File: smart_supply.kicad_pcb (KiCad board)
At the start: 2 copper layers, 40 x 40 mm, 26 parts, among them J2 Conn_01x05_Pin, J3 Conn_01x02_Pin, J4 Conn_01x06_Pin, J5 Conn_01x06_Pin, U5 ADE7953xCP, U7 MCP1825ST-3302E/DB, Y1 3.58M

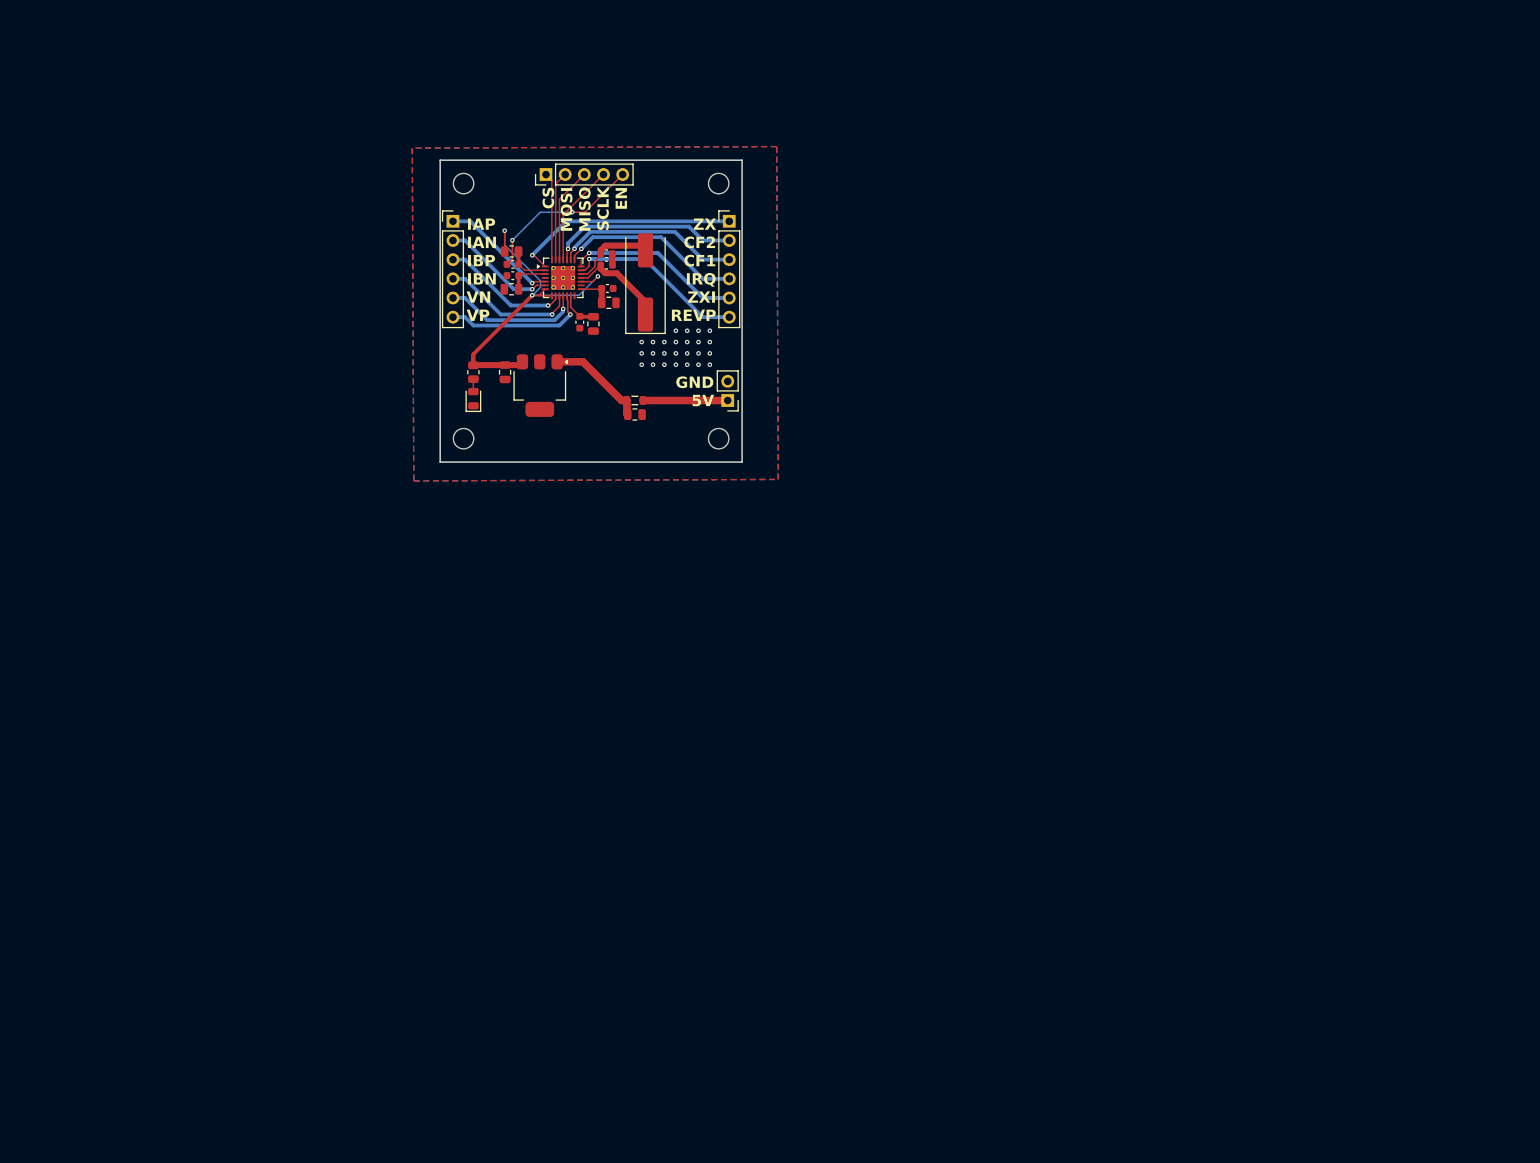
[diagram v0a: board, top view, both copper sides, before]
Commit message: created board
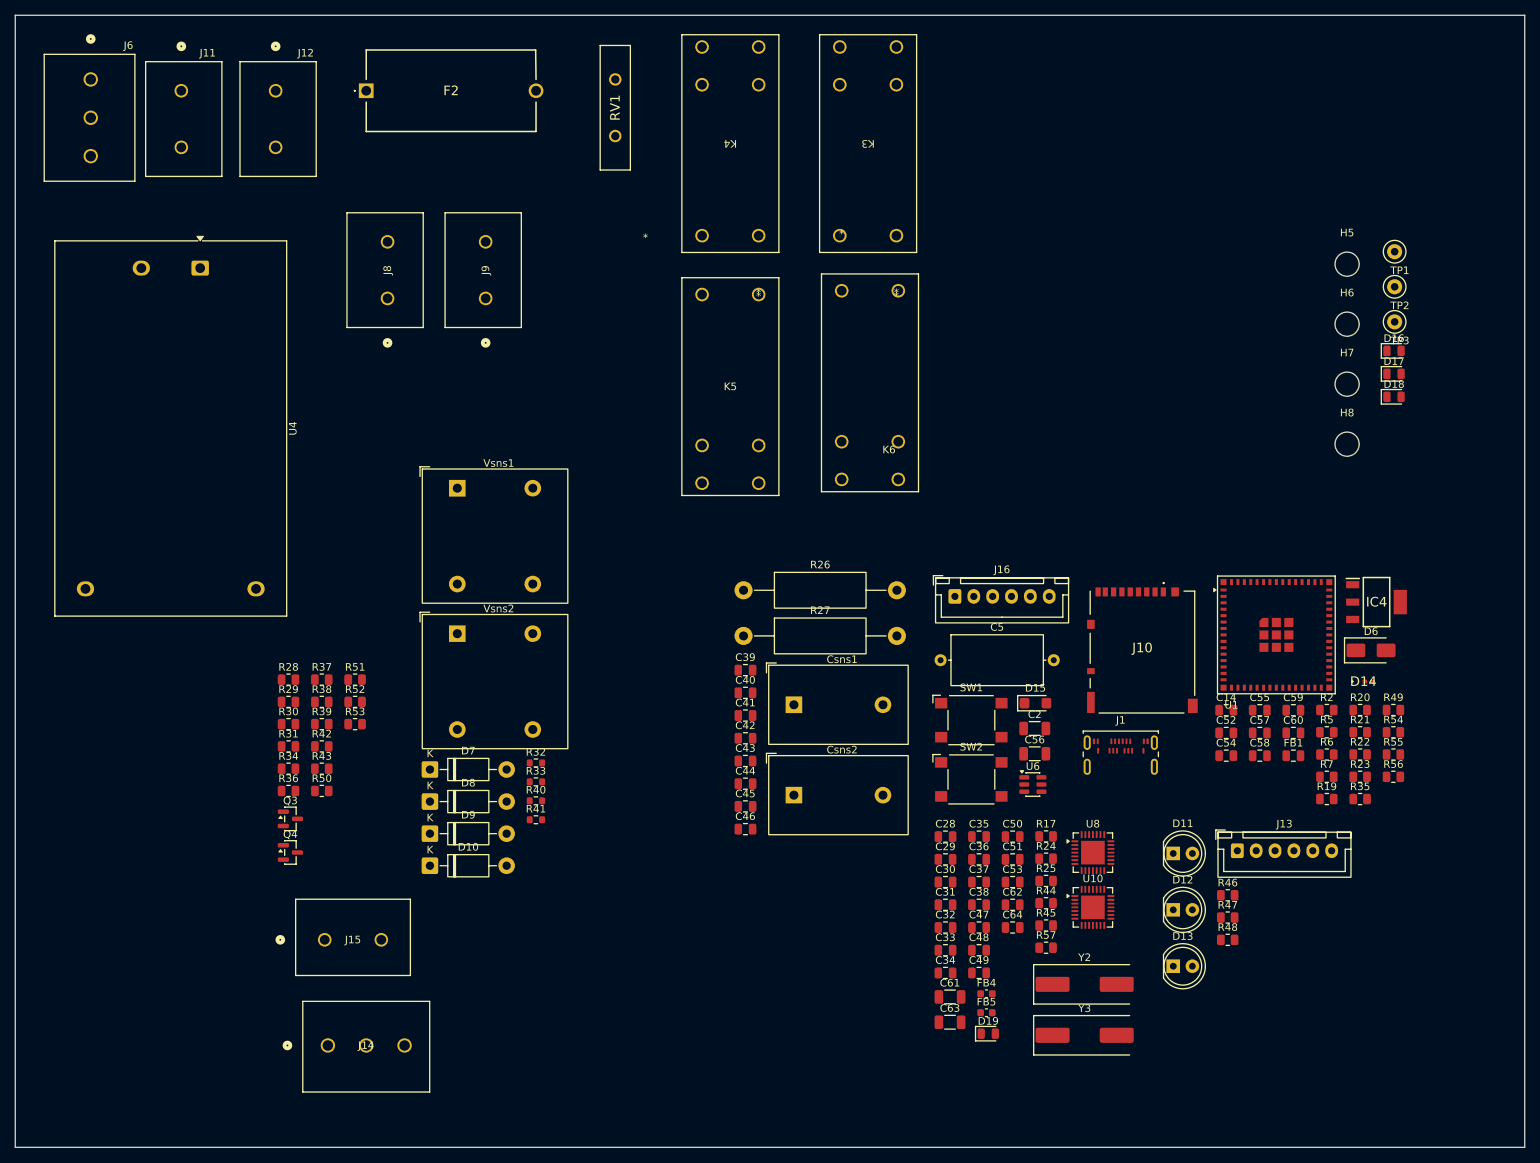
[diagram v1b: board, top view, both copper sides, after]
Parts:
- removed C15, C18: 20p, Capacitor_SMD:C_0603_1608Metric
- removed C19, C21, C24, C26: 100n, Capacitor_SMD:C_0603_1608Metric
- removed C20, C22, C23, C25: 4.7u, Capacitor_SMD:C_0805_2012Metric
- removed C27: 10u, Capacitor_SMD:C_0805_2012Metric
- removed D5: LED, LED_SMD:LED_0805_2012Metric
- removed FB2: FerriteBead_Small, Inductor_SMD:L_0805_2012Metric
- removed H1, H2, H3, H4: MountingHole, MountingHole:MountingHole_2.7mm_M2.5
- removed J2: Conn_01x05_Pin, Connector_PinHeader_2.54mm:PinHeader_1x05_P2.54mm_Vertical
- removed J3: Conn_01x02_Pin, Connector_PinHeader_2.54mm:PinHeader_1x02_P2.54mm_Vertical
- removed J4, J5: Conn_01x06_Pin, Connector_PinHeader_2.54mm:PinHeader_1x06_P2.54mm_Vertical
- removed R11: 10k, Resistor_SMD:R_0805_2012Metric
- removed R12: 50, Resistor_SMD:R_0805_2012Metric
- removed U5: ADE7953xCP, SmartSupplyLib:LFCSP-28-1EP_5x5mm_P0.5mm_EP3.14x3.14mm_ThermalVias
- removed U7: MCP1825ST-3302E/DB, Package_TO_SOT_SMD:SOT-223-3_TabPin2
- removed Y1: 3.58M, Crystal:Crystal_SMD_HC49-SD
- added C14: 10u, Capacitor_SMD:C_0805_2012Metric, F.Cu at (193.9, 106.6)
- added C2: 22u, Capacitor_SMD:C_1206_3216Metric, F.Cu at (168.6, 109.0)
- added C28: 4.7u, Capacitor_SMD:C_0805_2012Metric, F.Cu at (156.8, 123.3)
- added C29: 4.7u, Capacitor_SMD:C_0805_2012Metric, F.Cu at (156.8, 126.3)
- added C30: 100n, Capacitor_SMD:C_0805_2012Metric, F.Cu at (156.8, 129.3)
- added C31: 100n, Capacitor_SMD:C_0805_2012Metric, F.Cu at (156.8, 132.4)
- added C32: 4.7u, Capacitor_SMD:C_0805_2012Metric, F.Cu at (156.8, 135.4)
- added C33: 100n, Capacitor_SMD:C_0805_2012Metric, F.Cu at (156.8, 138.4)
- added C34: 100n, Capacitor_SMD:C_0805_2012Metric, F.Cu at (156.8, 141.4)
- added C35: 20p, Capacitor_SMD:C_0805_2012Metric, F.Cu at (161.2, 123.3)
- added C36: 20p, Capacitor_SMD:C_0805_2012Metric, F.Cu at (161.2, 126.3)
- added C37: 100n, Capacitor_SMD:C_0805_2012Metric, F.Cu at (161.2, 129.3)
- added C38: 100n, Capacitor_SMD:C_0805_2012Metric, F.Cu at (161.2, 132.4)
- added C39: 33n, Capacitor_SMD:C_0805_2012Metric, F.Cu at (130.2, 101.3)
- added C40: 33n, Capacitor_SMD:C_0805_2012Metric, F.Cu at (130.2, 104.3)
- added C41: 33n, Capacitor_SMD:C_0805_2012Metric, F.Cu at (130.2, 107.3)
- added C42: 33n, Capacitor_SMD:C_0805_2012Metric, F.Cu at (130.2, 110.3)
- added C43: 33n, Capacitor_SMD:C_0805_2012Metric, F.Cu at (130.2, 113.3)
- added C44: 33n, Capacitor_SMD:C_0805_2012Metric, F.Cu at (130.2, 116.3)
- added C45: 33n, Capacitor_SMD:C_0805_2012Metric, F.Cu at (130.2, 119.3)
- added C46: 33n, Capacitor_SMD:C_0805_2012Metric, F.Cu at (130.2, 122.3)
- added C47: 20p, Capacitor_SMD:C_0805_2012Metric, F.Cu at (161.2, 135.4)
- added C48: 20p, Capacitor_SMD:C_0805_2012Metric, F.Cu at (161.2, 138.4)
- added C49: 4.7u, Capacitor_SMD:C_0805_2012Metric, F.Cu at (161.2, 141.4)
- added C5: 220u, Capacitor_THT:C_Axial_L12.0mm_D6.5mm_P15.00mm_Horizontal, F.Cu at (156.1, 100.0)
- added C50: 4.7u, Capacitor_SMD:C_0805_2012Metric, F.Cu at (165.7, 123.3)
- added C51: 100n, Capacitor_SMD:C_0805_2012Metric, F.Cu at (165.7, 126.3)
- added C52: 100n, Capacitor_SMD:C_0805_2012Metric, F.Cu at (193.9, 109.6)
- added C53: 4.7u, Capacitor_SMD:C_0805_2012Metric, F.Cu at (165.7, 129.3)
- added C54: 100n, Capacitor_SMD:C_0805_2012Metric, F.Cu at (193.9, 112.6)
- added C55: 4.7u, Capacitor_SMD:C_0805_2012Metric, F.Cu at (198.4, 106.6)
- added C56: 10u, Capacitor_SMD:C_1206_3216Metric, F.Cu at (168.6, 112.3)
- added C57: 100n, Capacitor_SMD:C_0805_2012Metric, F.Cu at (198.4, 109.6)
- added C58: 100n, Capacitor_SMD:C_0805_2012Metric, F.Cu at (198.4, 112.6)
- added C59: 100n, Capacitor_SMD:C_0805_2012Metric, F.Cu at (202.8, 106.6)
- added C60: 100n, Capacitor_SMD:C_0805_2012Metric, F.Cu at (202.8, 109.6)
- added C61: 10u, Capacitor_SMD:C_1206_3216Metric, F.Cu at (157.3, 144.6)
- added C62: 100n, Capacitor_SMD:C_0805_2012Metric, F.Cu at (165.7, 132.4)
- added C63: 10u, Capacitor_SMD:C_1206_3216Metric, F.Cu at (157.3, 147.9)
- added C64: 100n, Capacitor_SMD:C_0805_2012Metric, F.Cu at (165.7, 135.4)
- added Csns1: ZMCT103C, Transformer_THT:Transformer_Zeming_ZMCT103C, F.Cu at (136.7, 105.9)
- added Csns2: ZMCT103C, Transformer_THT:Transformer_Zeming_ZMCT103C, F.Cu at (136.7, 117.8)
- added D10: 1N4007, Diode_THT:D_DO-41_SOD81_P10.16mm_Horizontal, F.Cu at (88.4, 127.2)
- added D11: LED, LED_THT:LED_D5.0mm, F.Cu at (186.9, 125.6)
- added D12: LED, LED_THT:LED_D5.0mm, F.Cu at (186.9, 133.0)
- added D13: LED, LED_THT:LED_D5.0mm, F.Cu at (186.9, 140.5)
- added D14: TPD1E10B06DPYR, SmartSupplyLib:TPD1E10B06DPYR, F.Cu at (212.8, 102.8)
- added D15: SMF5V0A, Diode_SMD:D_SMF, F.Cu at (168.7, 105.7)
- added D16: LED, LED_SMD:LED_0805_2012Metric, F.Cu at (216.2, 59.0)
- added D17: LED, LED_SMD:LED_0805_2012Metric, F.Cu at (216.2, 62.0)
- added D18: LED, LED_SMD:LED_0805_2012Metric, F.Cu at (216.2, 65.0)
- added D19: LED, LED_SMD:LED_0805_2012Metric, F.Cu at (162.4, 149.4)
- added D6: SS34, Diode_SMD:D_SMA, F.Cu at (213.1, 98.7)
- added D7: 1N4007, Diode_THT:D_DO-41_SOD81_P10.16mm_Horizontal, F.Cu at (88.4, 114.4)
- added D8: 1N4007, Diode_THT:D_DO-41_SOD81_P10.16mm_Horizontal, F.Cu at (88.4, 118.7)
- added D9: 1N4007, Diode_THT:D_DO-41_SOD81_P10.16mm_Horizontal, F.Cu at (88.4, 122.9)
- added F2: Fuse, SmartSupplyLib:fuse holder, F.Cu at (80.0, 24.5)
- added FB1: FerriteBead, Capacitor_SMD:C_0805_2012Metric, F.Cu at (202.8, 112.6)
- added FB4: FerriteBead, Capacitor_SMD:C_0603_1608Metric, F.Cu at (162.2, 144.2)
- added FB5: FerriteBead, Capacitor_SMD:C_0603_1608Metric, F.Cu at (162.2, 146.7)
- added H5: MountingHole, MountingHole:MountingHole_3.2mm_M3, F.Cu at (210.0, 47.5)
- added H6: MountingHole, MountingHole:MountingHole_3.2mm_M3, F.Cu at (210.0, 55.4)
- added H7: MountingHole, MountingHole:MountingHole_3.2mm_M3, F.Cu at (210.0, 63.4)
- added H8: MountingHole, MountingHole:MountingHole_3.2mm_M3, F.Cu at (210.0, 71.3)
- added IC4: MIC39100-3.3WS, SmartSupplyLib:SOT230P700X180-4N, F.Cu at (213.9, 92.2)
- added J1: USB_C_Receptacle_USB2.0_16P, Connector_USB:USB_C_Receptacle_Amphenol_124019772112A, F.Cu at (180.0, 113.9)
- added J10: DM3AT-SF-PEJM5, SmartSupplyLib:DM3ATSFPEJM5, F.Cu at (182.8, 98.3)
- added J11: 1717020, SmartSupplyLib:CONN_1717020_PXC, F.Cu at (55.5, 24.5)
- added J12: 1717020, SmartSupplyLib:CONN_1717020_PXC, F.Cu at (68.0, 24.5)
- added J13: Conn_01x06_Pin, Connector_JST:JST_XH_B6B-XH-A_1x06_P2.50mm_Vertical, F.Cu at (195.4, 125.2)
- added J14: 1730405, SmartSupplyLib:CONN_1730405_PXC, F.Cu at (74.9, 151.0)
- added J15: 1717020, SmartSupplyLib:CONN_1717020_PXC, F.Cu at (74.5, 137.0)
- added J16: Conn_01x06_Pin, Connector_JST:JST_XH_B6B-XH-A_1x06_P2.50mm_Vertical, F.Cu at (158.0, 91.5)
- added J6: 1730405, SmartSupplyLib:CONN_1730405_PXC, F.Cu at (43.5, 23.0)
- added J8: 1717020, SmartSupplyLib:CONN_1717020_PXC, F.Cu at (82.8, 52.0)
- added J9: 1717020, SmartSupplyLib:CONN_1717020_PXC, F.Cu at (95.8, 52.0)
- added K3: G2R-1A-E DC5, SmartSupplyLib:RELAY_G2R-1A-E AC12_OMR, F.Cu at (142.8, 19.3)
- added K4: G2R-1A-E DC5, SmartSupplyLib:RELAY_G2R-1A-E AC12_OMR, F.Cu at (124.5, 19.3)
- added K5: G2R-1A-E DC5, SmartSupplyLib:RELAY_G2R-1A-E AC12_OMR, F.Cu at (132.0, 75.9)
- added K6: G2R-1A-E DC5, SmartSupplyLib:RELAY_G2R-1A-E AC12_OMR, F.Cu at (150.5, 75.4)
- added Q3: AO3400A, Package_TO_SOT_SMD:SOT-23, F.Cu at (70.0, 121.0)
- added Q4: AO3400A, Package_TO_SOT_SMD:SOT-23, F.Cu at (70.0, 125.4)
- added R17: 10k, Resistor_SMD:R_0805_2012Metric, F.Cu at (170.1, 123.3)
- added R19: 10k, Resistor_SMD:R_0805_2012Metric, F.Cu at (207.3, 118.3)
- added R2: 0, Resistor_SMD:R_0805_2012Metric, F.Cu at (207.3, 106.5)
- added R20: 10k, Resistor_SMD:R_0805_2012Metric, F.Cu at (211.7, 106.5)
- added R21: 10k, Resistor_SMD:R_0805_2012Metric, F.Cu at (211.7, 109.5)
- added R22: 10k, Resistor_SMD:R_0805_2012Metric, F.Cu at (211.7, 112.5)
- added R23: 10k, Resistor_SMD:R_0805_2012Metric, F.Cu at (211.7, 115.4)
- added R24: 10k, Resistor_SMD:R_0805_2012Metric, F.Cu at (170.1, 126.2)
- added R25: 10k, Resistor_SMD:R_0805_2012Metric, F.Cu at (170.1, 129.2)
- added R26: 47k, Resistor_THT:R_Axial_DIN0414_L11.9mm_D4.5mm_P20.32mm_Horizontal, F.Cu at (130.0, 90.7)
- added R27: 47k, Resistor_THT:R_Axial_DIN0414_L11.9mm_D4.5mm_P20.32mm_Horizontal, F.Cu at (130.0, 96.7)
- added R28: 100, Resistor_SMD:R_0805_2012Metric, F.Cu at (69.7, 102.5)
- added R29: 1k, Resistor_SMD:R_0805_2012Metric, F.Cu at (69.7, 105.5)
- added R30: 1k, Resistor_SMD:R_0805_2012Metric, F.Cu at (69.7, 108.4)
- added R31: 1k, Resistor_SMD:R_0805_2012Metric, F.Cu at (69.7, 111.4)
- added R32: 10, Resistor_SMD:R_0603_1608Metric, F.Cu at (102.5, 113.6)
- added R33: 10, Resistor_SMD:R_0603_1608Metric, F.Cu at (102.5, 116.1)
- added R34: 1k, Resistor_SMD:R_0805_2012Metric, F.Cu at (69.7, 114.3)
- added R35: 1.5k, Resistor_SMD:R_0805_2012Metric, F.Cu at (211.7, 118.3)
- added R36: 20k, Resistor_SMD:R_0805_2012Metric, F.Cu at (69.7, 117.3)
- added R37: 1k, Resistor_SMD:R_0805_2012Metric, F.Cu at (74.1, 102.5)
- added R38: 100, Resistor_SMD:R_0805_2012Metric, F.Cu at (74.1, 105.5)
- added R39: 1k, Resistor_SMD:R_0805_2012Metric, F.Cu at (74.1, 108.4)
- added R40: 33, Resistor_SMD:R_0603_1608Metric, F.Cu at (102.5, 118.6)
- added R41: 33, Resistor_SMD:R_0603_1608Metric, F.Cu at (102.5, 121.1)
- added R42: 1k, Resistor_SMD:R_0805_2012Metric, F.Cu at (74.1, 111.4)
- added R43: 1k, Resistor_SMD:R_0805_2012Metric, F.Cu at (74.1, 114.3)
- added R44: 10k, Resistor_SMD:R_0805_2012Metric, F.Cu at (170.1, 132.2)
- added R45: 10k, Resistor_SMD:R_0805_2012Metric, F.Cu at (170.1, 135.1)
- added R46: 270, Resistor_SMD:R_0805_2012Metric, F.Cu at (194.2, 131.1)
- added R47: 270, Resistor_SMD:R_0805_2012Metric, F.Cu at (194.2, 134.1)
- added R48: 270, Resistor_SMD:R_0805_2012Metric, F.Cu at (194.2, 137.0)
- added R49: 10k, Resistor_SMD:R_0805_2012Metric, F.Cu at (216.1, 106.5)
- added R5: 10k, Resistor_SMD:R_0805_2012Metric, F.Cu at (207.3, 109.5)
- added R50: 100, Resistor_SMD:R_0805_2012Metric, F.Cu at (74.1, 117.3)
- added R51: 100k, Resistor_SMD:R_0805_2012Metric, F.Cu at (78.5, 102.5)
- added R52: 100, Resistor_SMD:R_0805_2012Metric, F.Cu at (78.5, 105.5)
- added R53: 100k, Resistor_SMD:R_0805_2012Metric, F.Cu at (78.5, 108.4)
- added R54: 470, Resistor_SMD:R_0805_2012Metric, F.Cu at (216.1, 109.5)
- added R55: 470, Resistor_SMD:R_0805_2012Metric, F.Cu at (216.1, 112.5)
- added R56: 470, Resistor_SMD:R_0805_2012Metric, F.Cu at (216.1, 115.4)
- added R57: 470, Resistor_SMD:R_0805_2012Metric, F.Cu at (170.1, 138.1)
- added R6: 5.1k, Resistor_SMD:R_0805_2012Metric, F.Cu at (207.3, 112.5)
- added R7: 5.1k, Resistor_SMD:R_0805_2012Metric, F.Cu at (207.3, 115.4)
- added RV1: MOV-14D241K, SmartSupplyLib:MOV14D241K, F.Cu at (113.0, 30.5)
- added SW1: SW_Push, Button_Switch_SMD:SW_SPST_Omron_B3FS-100xP, F.Cu at (160.2, 107.9)
- added SW2: SW_Push, Button_Switch_SMD:SW_SPST_Omron_B3FS-100xP, F.Cu at (160.2, 115.8)
- added TP1: TestPoint, TestPoint:TestPoint_Loop_D2.50mm_Drill1.0mm, F.Cu at (216.3, 45.8)
- added TP2: TestPoint, TestPoint:TestPoint_Loop_D2.50mm_Drill1.0mm, F.Cu at (216.3, 50.5)
- added TP3: TestPoint, TestPoint:TestPoint_Loop_D2.50mm_Drill1.0mm, F.Cu at (216.3, 55.1)
- added U1: ESP32-S3-MINI-1U, RF_Module:ESP32-S2-MINI-1U, F.Cu at (200.6, 96.6)
- added U10: ADE7953xCP, Package_CSP:LFCSP-28-1EP_5x5mm_P0.5mm_EP3.14x3.14mm, F.Cu at (176.3, 132.7)
- added U4: HLK-10M05, Converter_ACDC:Converter_ACDC_Hi-Link_HLK-10Mxx, F.Cu at (58.0, 48.0)
- added U6: USBLC6-2SC6, Package_TO_SOT_SMD:SOT-23-6, F.Cu at (168.3, 116.4)
- added U8: ADE7953xCP, Package_CSP:LFCSP-28-1EP_5x5mm_P0.5mm_EP3.14x3.14mm, F.Cu at (176.3, 125.5)
- added Vsns1: ZMPT101K, Transformer_THT:Transformer_Zeming_ZMPT101K, F.Cu at (92.1, 77.2)
- added Vsns2: ZMPT101K, Transformer_THT:Transformer_Zeming_ZMPT101K, F.Cu at (92.1, 96.4)
- added Y2: 3.58M, Crystal:Crystal_SMD_HC49-SD, F.Cu at (175.2, 142.9)
- added Y3: 3.58M, Crystal:Crystal_SMD_HC49-SD, F.Cu at (175.2, 149.7)
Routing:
- net +3.3V: track 51.8 -> 0.00 mm, vias 3 -> 0
- net /ADE Module/ZX: track 30.3 -> 0.00 mm, vias 1 -> 0
- net /ADE Module/CF2: track 25.3 -> 0.00 mm, vias 1 -> 0
- net /ADE Module/CF1: track 24.7 -> 0.00 mm, vias 1 -> 0
- net /ADE Module/IRQ: track 24.4 -> 0.00 mm, vias 1 -> 0
- net /ADE Module/REVP: track 24.0 -> 0.00 mm, vias 1 -> 0
- net /ADE Module/ZX_I: track 23.3 -> 0.00 mm, vias 1 -> 0
- net /ADE Module/EN: track 21.7 -> 0.00 mm, vias 2 -> 0
- net /ADE Module/VP: track 19.3 -> 0.00 mm, vias 1 -> 0
- net /ADE Module/VN: track 18.4 -> 0.00 mm, vias 1 -> 0
- net /ADE Module/IBN: track 18.0 -> 0.00 mm, vias 1 -> 0
- net /ADE Module/IBP: track 16.9 -> 0.00 mm, vias 1 -> 0
- net /ADE Module/IAP: track 15.7 -> 0.00 mm, vias 1 -> 0
- net /ADE Module/IAN: track 15.1 -> 0.00 mm, vias 1 -> 0
- net /ADE Module/CLKIN: track 13.6 -> 0.00 mm
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- removed copper zone on B.Cu, net GND
- removed copper zone on F.Cu, net GND
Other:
- board size 40 x 40 mm -> 200 x 150 mm
- board text removed: "ADE7953 Breakout Board"
- board text removed: "CS MOSI MISO SCLK EN"
- board text removed: "GND 5V"
- board text removed: "IAP IAN IBP IBN VN VP"
- board text removed: "ZX CF2 CF1 IRQ ZXI REVP"
